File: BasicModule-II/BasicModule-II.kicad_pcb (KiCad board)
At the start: 2 copper layers, 17.8 x 20.3 mm, 12 parts, among them M1 LED_PIRANHA_5MM, P1 CONN_01X03, Q1 Q_NPN_BCE

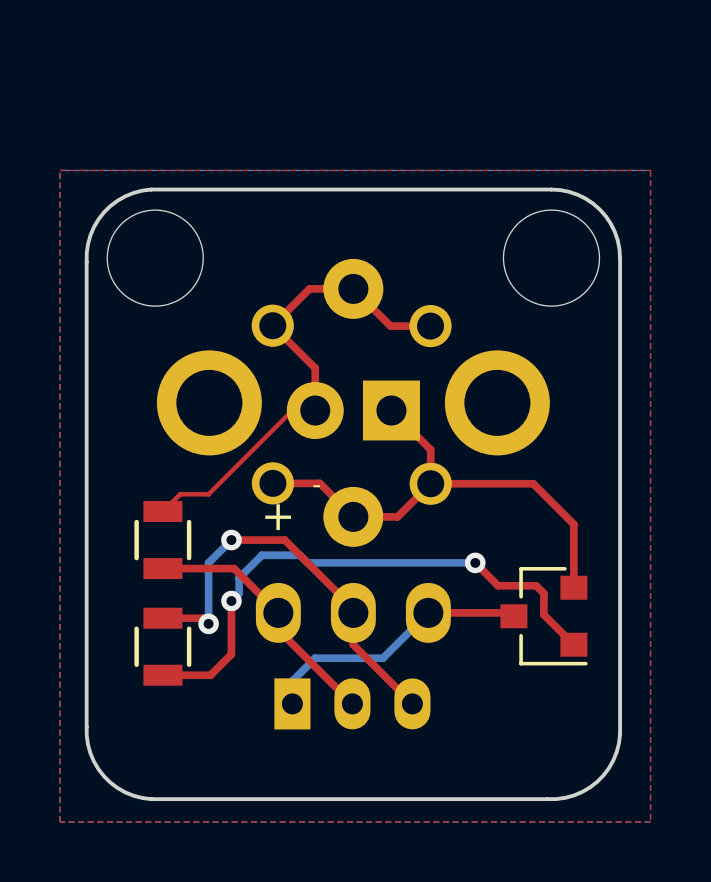
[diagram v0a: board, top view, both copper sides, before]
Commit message: LAyout terminado
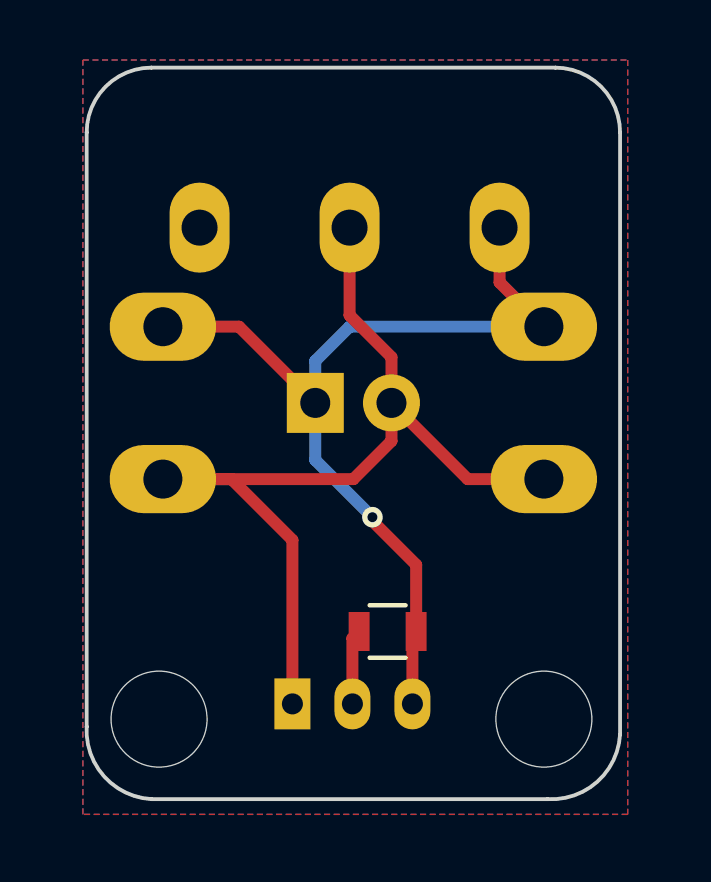
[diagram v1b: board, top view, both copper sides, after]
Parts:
- removed BZ1: Buzzer, Buzzers_Beepers:Buzzer_12x9.5RM7.6
- removed D1: LED, LEDs:LED-5MM
- removed G***: LOGO, logos_frizzy:web
- removed G***: LOGO, logos_frizzy:glance
- removed M1: LED_PIRANHA_5MM, SparkFun-LED:LED_PIRANHA_5MM
- removed Q1: Q_NPN_BCE, TO_SOT_Packages_SMD:SOT-23
- removed the REF** at (131.3, 96.5)
- removed the REF** at (144.5, 96.5)
- removed RV1: POT, w_pth_resistors:trimmer_alps-rk09k1130ah1
- added REF**: MountingHole_3.2mm_M3, Mounting_Holes:MountingHole_3.2mm_M3, F.Cu at (144.3, 111.9)
- added REF**: MountingHole_3.2mm_M3, Mounting_Holes:MountingHole_3.2mm_M3, F.Cu at (131.4, 111.9)
- added SW1: Pulsador, Buttons_Switches_THT:SW_PUSH-12mm, F.Cu at (137.9, 101.3)
- added SW2: Final_carrera, frizzy_switches:limit_sw_tiaihua, F.Cu at (137.8, 95.5)
- R1: value 1k -> 10k
- R2: value 1k -> R_PHOTO; footprint Resistors_SMD:R_0805 -> LEDs:LED-5MM
- moved R1 7.51 mm to (139.1, 109.0), turned to 0 degrees
- moved R2 6.83 mm to (136.7, 101.3), turned to 0 degrees
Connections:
- P1 pad 2: +5V -> 5V
- R1 pad 1: SIGNAL -> 5V
- R1 pad 2: Net-(Q1-Pad1) -> SIGNAL
- R2 pad 1: Net-(BZ1-Pad2) -> SIGNAL
- R2 pad 2: +5V -> GND
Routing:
- net GND: track 9.13 -> 33.2 mm
- net Net-(Q1-Pad1): track 18.3 -> 0.00 mm, vias 2 -> 0
- net SIGNAL: track 13.7 -> 31.2 mm, vias 2 -> 1
- net Net-(BZ1-Pad1): track 16.6 -> 0.00 mm
- net Net-(BZ1-Pad2): track 16.2 -> 0.00 mm
- net +5V: track 9.49 -> 0.00 mm
- net 5V: track 0.00 -> 2.98 mm
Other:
- board size 17.8 x 20.3 mm -> 17.8 x 24.4 mm
